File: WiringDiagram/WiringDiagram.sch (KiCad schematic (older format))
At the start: 9 parts

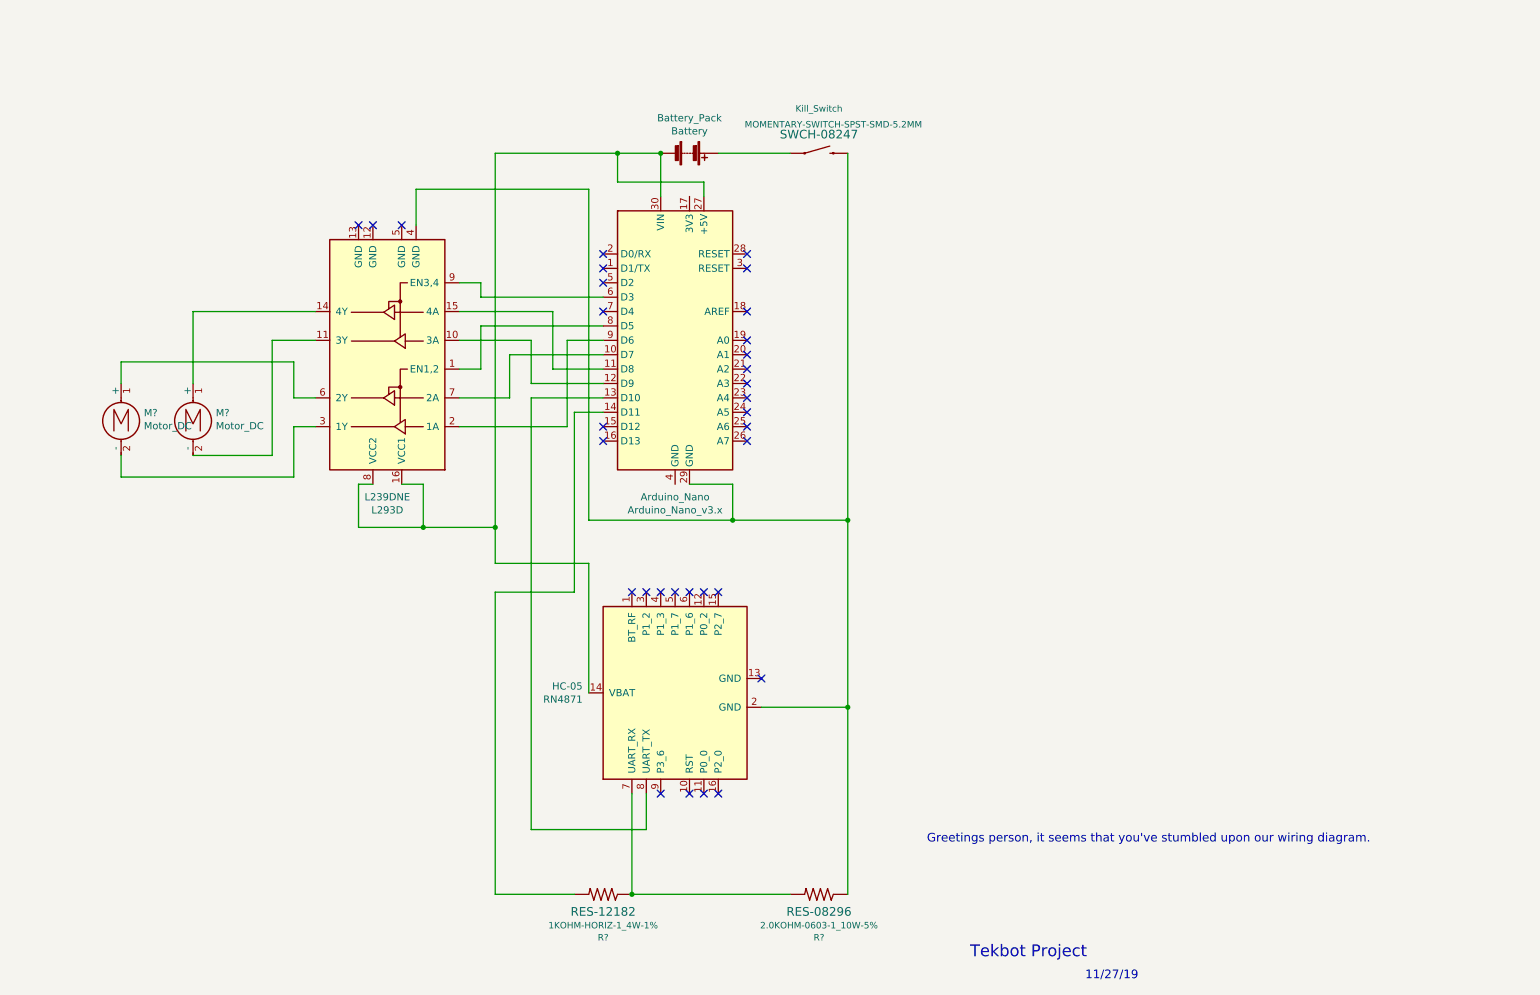
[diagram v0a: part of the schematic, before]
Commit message: Add files via upload
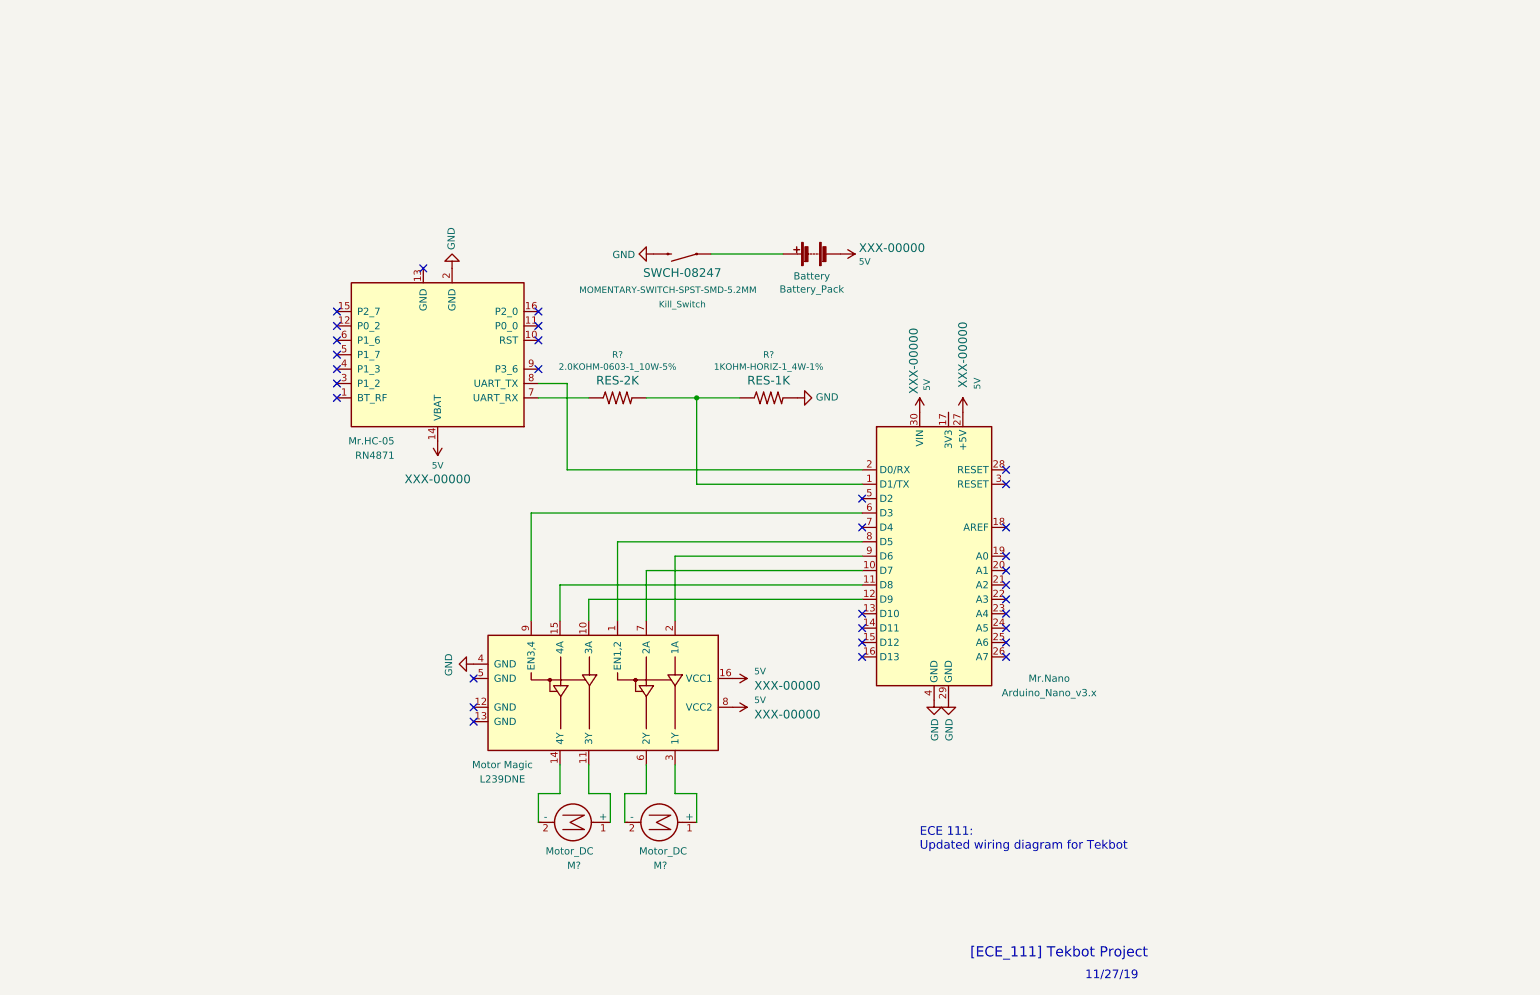
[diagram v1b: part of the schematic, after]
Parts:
- L239DNE: value L293D -> Motor Magic
- R?: Field4 RES-12182 -> RES-1K
- R?: Field4 RES-08296 -> RES-2K
- renumbered HC-05 to Mr.HC-05, Arduino_Nano to Mr.Nano
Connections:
- net at Mr.Nano.1 (D1/TX): now also R?.2, R?.P$1 (1)
- net at Mr.Nano.13 (D10): no longer Mr.HC-05.8 (UART_TX)
- net at Mr.Nano.14 (D11): no longer R?.P$2 (2)
- net at Mr.Nano.2 (D0/RX): now also Mr.HC-05.8 (UART_TX)
- net 5V: now reaches Battery_Pack.2 (-), L239DNE.16 (VCC1), L239DNE.8 (VCC2), Mr.HC-05.14 (VBAT), Mr.Nano.27 (+5V), Mr.Nano.30 (VIN)
- net GND: now reaches Kill_Switch.3 (2), L239DNE.4 (GND), Mr.HC-05.2 (GND), Mr.Nano.29 (GND)
- net GND: now also Mr.Nano.4 (GND), R?.P$2 (2); no longer R?.1
- net at L239DNE.11 (3Y): now also M?.1 (+); no longer M?.2 (-)
- net at L239DNE.14 (4Y): now also M?.2 (-); no longer M?.1 (+)
- net at L239DNE.3 (1Y): now also M?.1 (+); no longer M?.2 (-)
- net at L239DNE.6 (2Y): now also M?.2 (-); no longer M?.1 (+)
- new net: Mr.HC-05.7 (UART_RX), R?.1
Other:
- note added: "ECE 111: \nUpdated wiring diagram for Tekbot\n"
- note added: "[ECE_111] Tekbot Project\n"
- note removed: "Greetings person, it seems that you've stumbled upon our wiring diagram. \n"
- note removed: "Tekbot Project\n"
- moved on the sheet: Battery_Pack, Kill_Switch, L239DNE, M?, Mr.HC-05, Mr.Nano, R?
